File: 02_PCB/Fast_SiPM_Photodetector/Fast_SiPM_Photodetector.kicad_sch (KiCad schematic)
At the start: 7 parts, among them J1 PTSM 0,5/ 2-HH-2,5-SMD R32, J2 SMA, J3 PTSM 0,5/ 4-HH-2,5-SMD R32

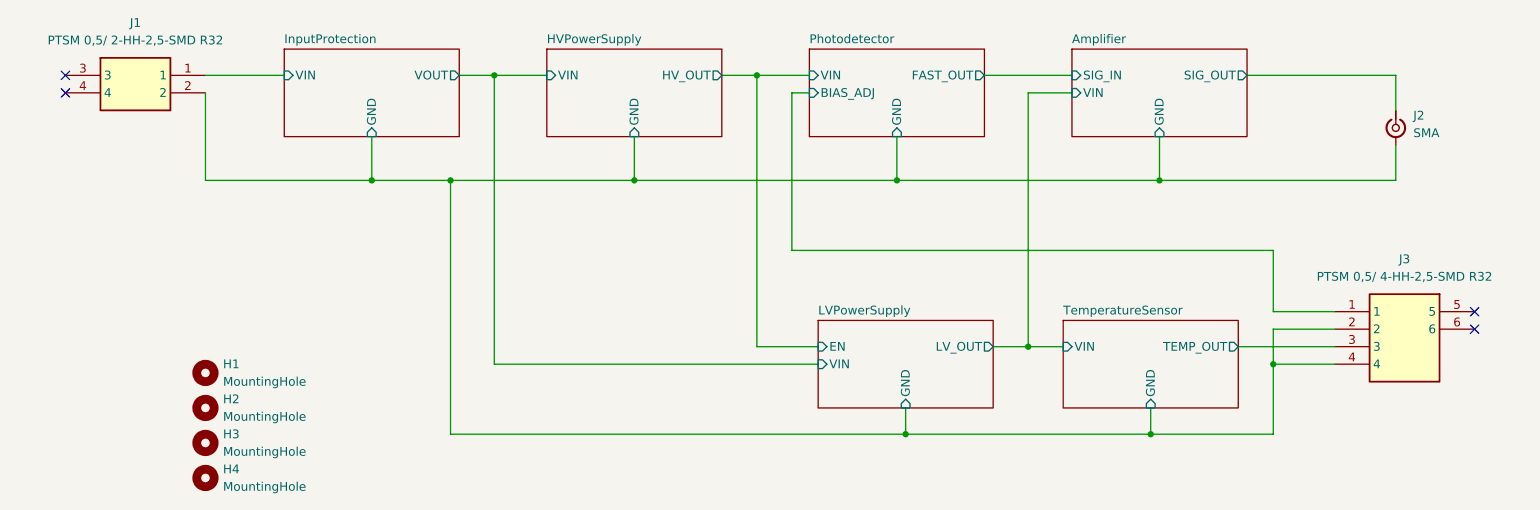
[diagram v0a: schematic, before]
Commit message: feat(detector): update schematic and pcb after first prototype
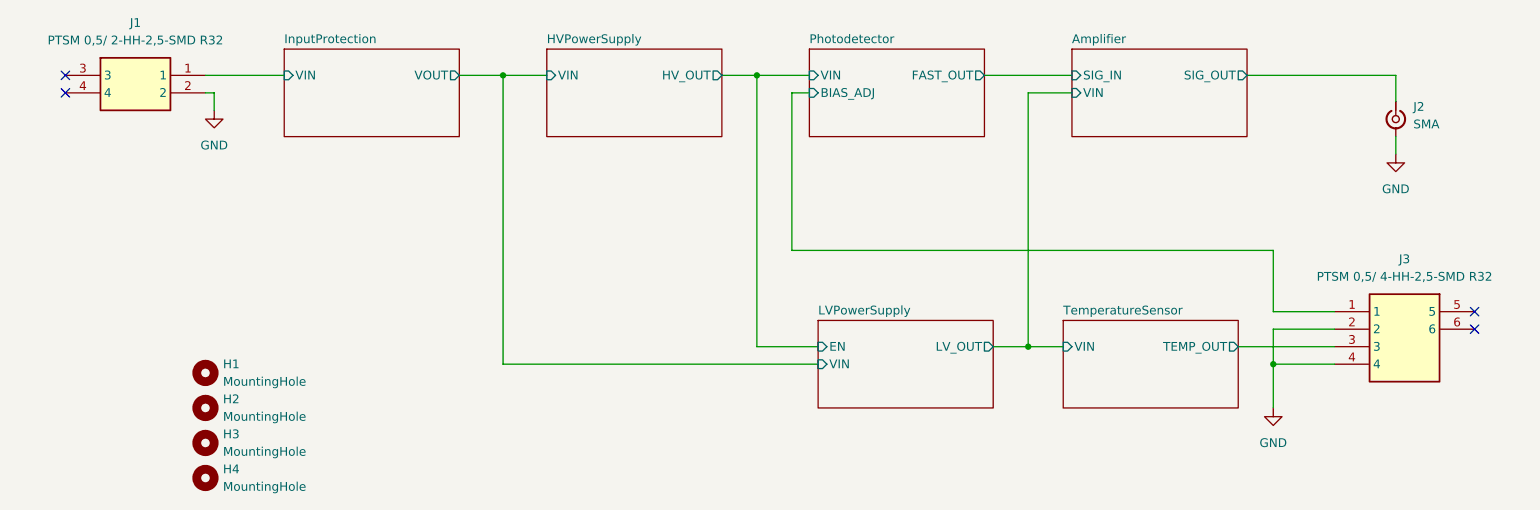
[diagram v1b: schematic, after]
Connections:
- net Amplifier/GND renamed GND
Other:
- sheet Amplifier ports: added none; removed GND
- sheet HVPowerSupply ports: added none; removed GND
- sheet InputProtection ports: added none; removed GND
- sheet LVPowerSupply ports: added none; removed GND
- sheet Photodetector ports: added none; removed GND
- sheet TemperatureSensor ports: added none; removed GND
- moved on the sheet: J2
